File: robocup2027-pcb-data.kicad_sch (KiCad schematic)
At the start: 40 parts, among them M5 Motor_Servo, M6 Motor_Servo, Q1 BPW40, Q2 BPW40, U1 ESP32-DEVKITC-32E

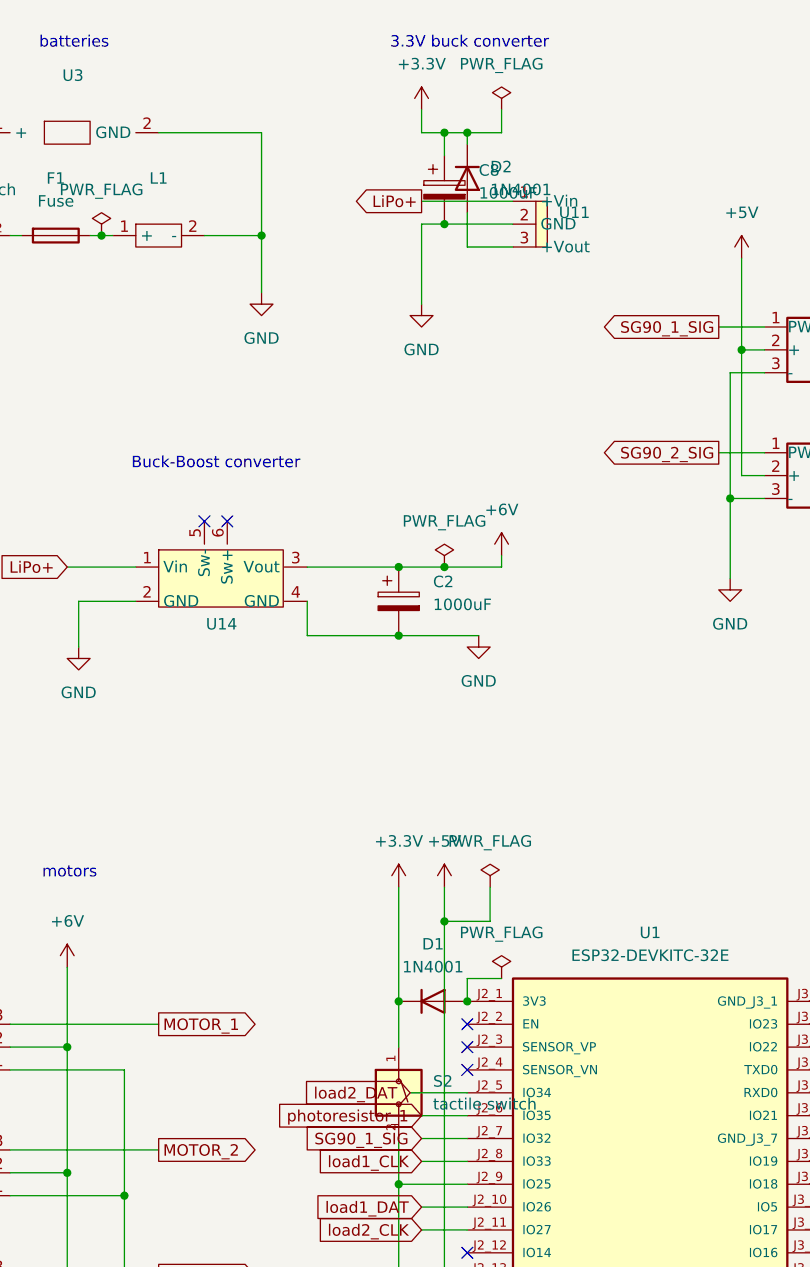
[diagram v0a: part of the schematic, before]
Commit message: update library
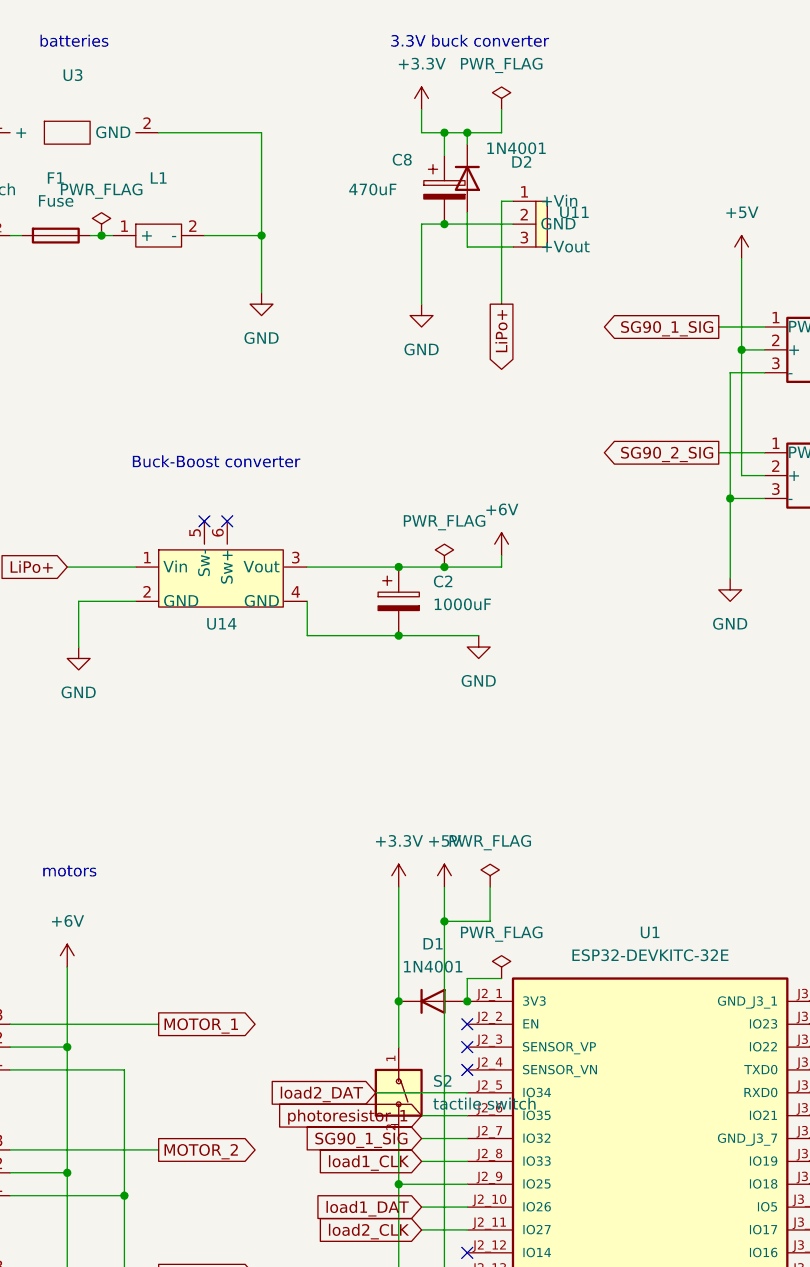
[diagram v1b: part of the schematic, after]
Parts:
- C1, C3, C4, C5, C6, C7: footprint (none) -> robo:2.54mm_capacitor
- C2: footprint (none) -> robo:5.08mm_capacitor_1
- C8: value 1000uF -> 470uF; footprint (none) -> robo:5.08mm_capacitor_1
- L1: footprint (none) -> robo:LiPo
- M5, M6: footprint (none) -> robo:servo_motor_3
- U3: footprint (none) -> robo:voltmeter
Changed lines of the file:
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@@
 	(wire
 		(pts
-			(xy 87.63 133.35) (xy 93.98 133.35)
+			(xy 83.82 133.35) (xy 93.98 133.35)
 		)
 		(stroke
@@
 	(wire
 		(pts
-			(xy 88.9 34.29) (xy 99.06 34.29)
+			(xy 97.79 45.72) (xy 97.79 34.29)
 		)
 		(stroke
@@
 	(wire
 		(pts
+			(xy 97.79 34.29) (xy 99.06 34.29)
+		)
+		(stroke
+			(width 0)
+			(type default)
+		)
+	)
+	(wire
+		(pts
 			(xy 91.44 114.3) (xy 91.44 168.91)
 		)
@@
 	(global_label "load2_DAT"
 		(shape input)
-		(at 87.63 133.35 180)
+		(at 83.82 133.35 180)
 		(fields_autoplaced yes)
 		(effects
@@
 		)
 		(property "Intersheetrefs" "${INTERSHEET_REFS}"
-			(at 75.0293 133.35 0)
+			(at 71.2193 133.35 0)
 			(effects
 				(font
@@
 	(global_label "LiPo+"
 		(shape output)
-		(at 88.9 34.29 180)
+		(at 97.79 45.72 270)
 		(fields_autoplaced yes)
 		(effects
@@
 		)
 		(property "Intersheetrefs" "${INTERSHEET_REFS}"
-			(at 80.2905 34.29 0)
+			(at 97.79 54.3295 90)
 			(effects
 				(font
@@
 			)
 		)
-		(property "Footprint" ""
+		(property "Footprint" "robo:voltmeter"
 			(at 49.53 26.67 0)
 			(effects
@@
 			)
 		)
-		(property "Footprint" ""
+		(property "Footprint" "robo:5.08mm_capacitor_1"
 			(at 87.3252 82.55 0)
 			(effects
@@
 			)
 		)
-		(property "Footprint" ""
+		(property "Footprint" "robo:servo_motor_3"
 			(at 134.62 55.626 0)
 			(effects
@@
 			)
 		)
-		(property "Footprint" ""
+		(property "Footprint" "robo:2.54mm_capacitor"
 			(at 176.2252 118.11 0)
 			(effects
@@
 			)
 		)
-		(property "Footprint" ""
+		(property "Footprint" "robo:LiPo"
 			(at 59.69 38.1 0)
 			(effects
@@
 			)
 		)
-		(property "Footprint" ""
+		(property "Footprint" "robo:servo_motor_3"
 			(at 134.62 69.596 0)
 			(effects
@@
 			)
 		)
-		(property "Footprint" ""
+		(property "Footprint" "robo:2.54mm_capacitor"
 			(at 176.2252 41.91 0)
 			(effects
@@
 			)
 		)
-		(property "Footprint" ""
+		(property "Footprint" "robo:2.54mm_capacitor"
 			(at 176.2252 60.96 0)
 			(effects
@@
 		(on_board yes)
 		(dnp no)
-		(fields_autoplaced yes)
 		(property "Reference" "C8"
-			(at 95.25 30.8609 0)
+			(at 85.598 29.718 0)
 			(effects
 				(font
@@
 			)
 		)
-		(property "Value" "1000uF"
-			(at 95.25 33.4009 0)
+		(property "Value" "470uF"
+			(at 80.772 33.02 0)
 			(effects
 				(font
@@
 			)
 		)
-		(property "Footprint" ""
+		(property "Footprint" "robo:5.08mm_capacitor_1"
 			(at 92.4052 36.83 0)
 			(effects
@@
 			)
 		)
-		(property "Footprint" ""
+		(property "Footprint" "robo:2.54mm_capacitor"
 			(at 176.2252 80.01 0)
 			(effects
@@
 			)
 		)
-		(property "Footprint" ""
+		(property "Footprint" "robo:2.54mm_capacitor"
 			(at 176.2252 137.16 0)
 			(effects
@@
 			)
 		)
-		(property "Footprint" ""
+		(property "Footprint" "robo:2.54mm_capacitor"
 			(at 176.2252 99.06 0)
 			(effects
@@
 		(on_board yes)
 		(dnp no)
-		(fields_autoplaced yes)
 		(property "Reference" "D2"
-			(at 96.52 30.4799 90)
+			(at 98.806 29.972 90)
 			(effects
 				(font
@@
 		)
 		(property "Value" "1N4001"
-			(at 96.52 33.0199 90)
+			(at 96.012 28.448 90)
 			(effects
 				(font

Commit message: update
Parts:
- F1: footprint (none) -> robo:5.08mm_capacitor_1
- R1, R2, R3, R4, R5: footprint (none) -> robo:Resister
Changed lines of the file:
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@@
 			)
 		)
-		(property "Footprint" ""
+		(property "Footprint" "robo:Resister"
 			(at 235.712 48.26 90)
 			(effects
@@
 			)
 		)
-		(property "Footprint" ""
+		(property "Footprint" "robo:Resister"
 			(at 143.002 128.27 90)
 			(effects
@@
 			)
 		)
-		(property "Footprint" ""
+		(property "Footprint" "robo:5.08mm_capacitor_1"
 			(at 48.26 36.322 90)
 			(effects
@@
 			)
 		)
-		(property "Footprint" ""
+		(property "Footprint" "robo:Resister"
 			(at 242.062 59.69 90)
 			(effects
@@
 			)
 		)
-		(property "Footprint" ""
+		(property "Footprint" "robo:Resister"
 			(at 84.582 163.83 90)
 			(effects
@@
 			)
 		)
-		(property "Footprint" ""
+		(property "Footprint" "robo:Resister"
 			(at 150.622 124.46 90)
 			(effects
